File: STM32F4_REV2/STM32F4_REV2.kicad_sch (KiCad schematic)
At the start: 50 parts, among them IC1 MP2359DJ-LF-Z, J1 Screw_Terminal_01x02, J2 SWD, J3 Conn_01x04, J4 Conn_01x04, J5 USB_B_Micro, Q1 AO3401A, SW1 SW_SPDT, U1 STM32F405RGT6, U2 USBLC6-2SC6, Y1 16MHz

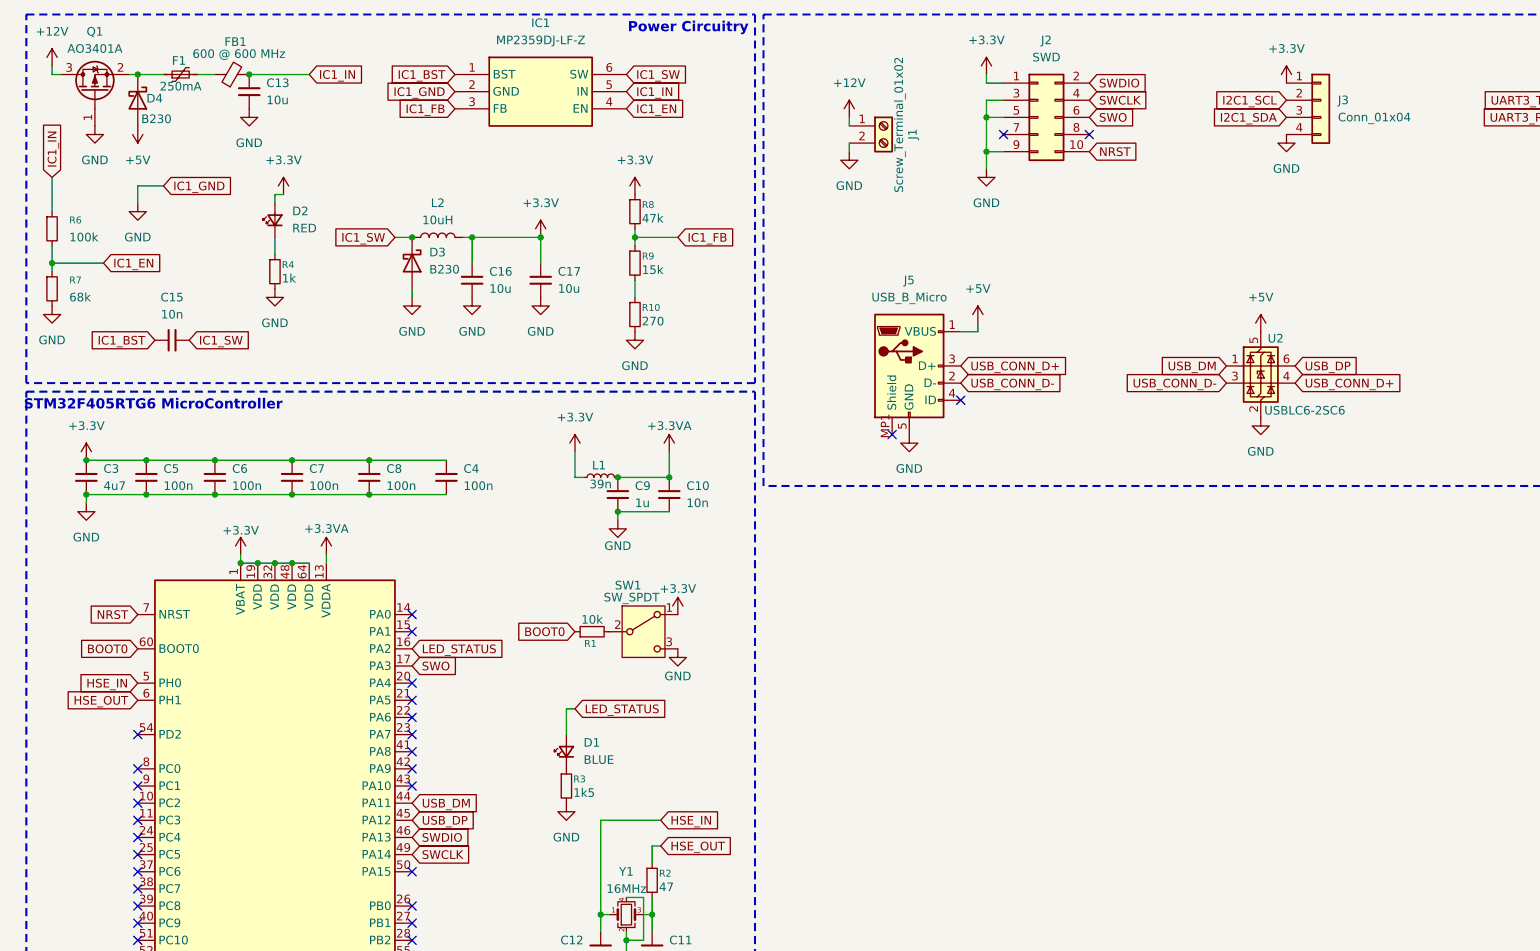
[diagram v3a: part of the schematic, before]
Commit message: Uploading the PCB files
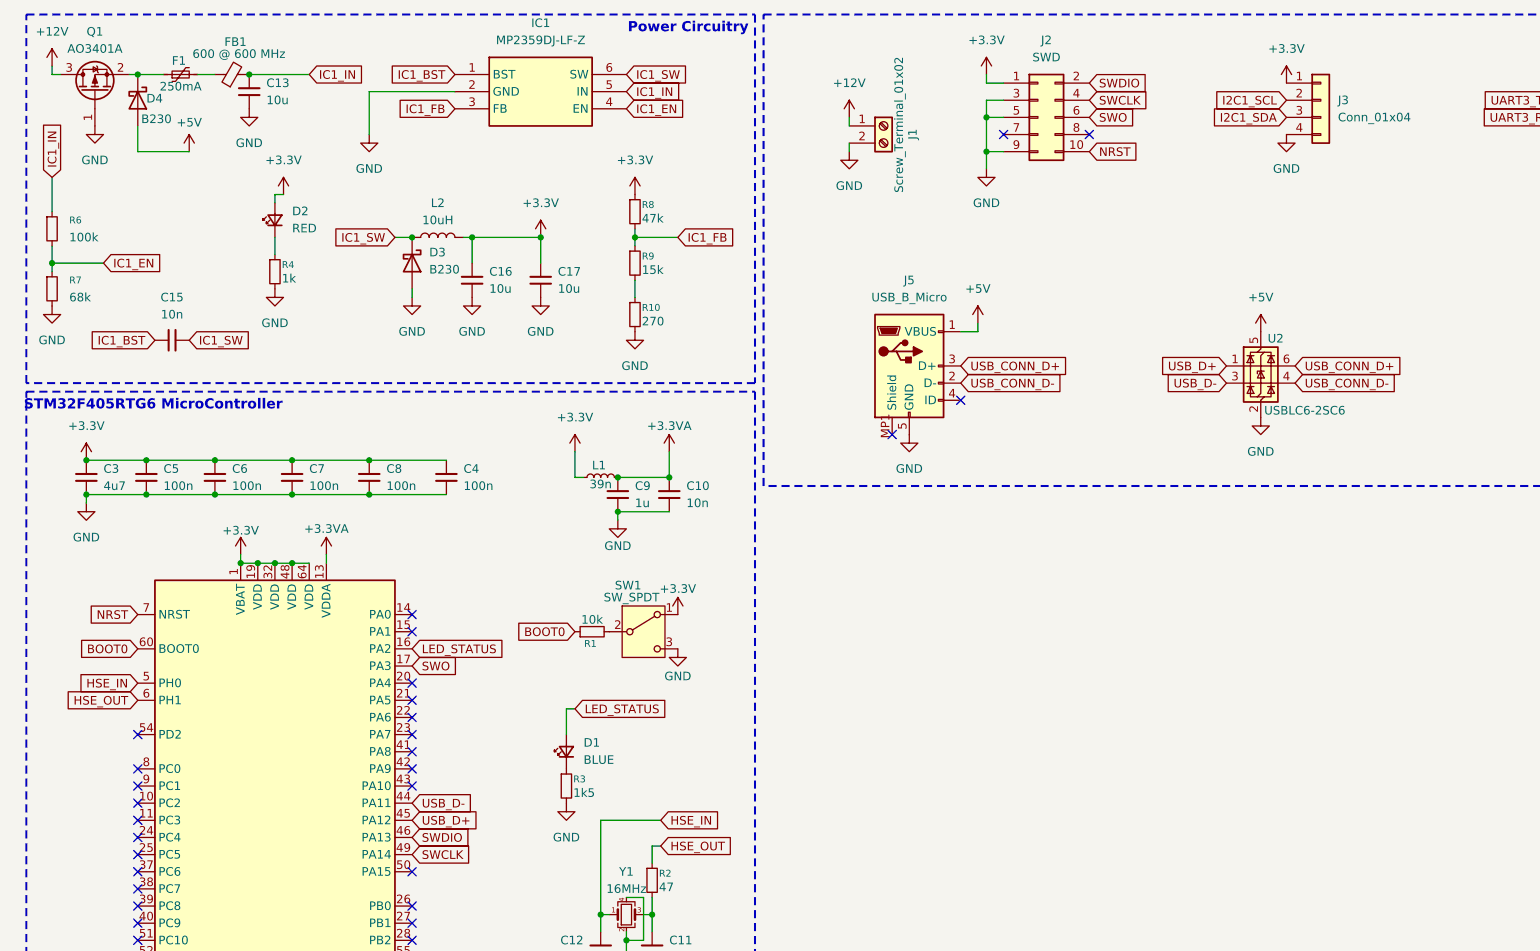
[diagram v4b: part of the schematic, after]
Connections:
- net USB_CONN_D+: now also U2.6 (I/O1); no longer U2.4 (I/O2)
- net USB_CONN_D-: now also U2.4 (I/O2); no longer U2.3 (I/O2)
- net USB_DM renamed USB_D+
- net USB_D+: now also U1.45 (PA12); no longer U1.44 (PA11)
- removed net USB_DP: U1.45 (PA12), U2.6 (I/O1)
- new net USB_D-: U1.44 (PA11), U2.3 (I/O2)
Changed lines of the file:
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@@
 	(wire
 		(pts
+			(xy 36.83 33.02) (xy 29.21 33.02)
+		)
+		(stroke
+			(width 0)
+			(type default)
+		)
+	)
+	(wire
+		(pts
 			(xy 101.6 182.88) (xy 101.6 191.77)
 		)
@@
 	(wire
 		(pts
-			(xy 29.21 38.1) (xy 29.21 40.64)
+			(xy 63.5 24.13) (xy 63.5 30.48)
 		)
 		(stroke
@@
 	(wire
 		(pts
-			(xy 33.02 38.1) (xy 29.21 38.1)
+			(xy 63.5 24.13) (xy 76.2 24.13)
 		)
 		(stroke
@@
 	(wire
 		(pts
+			(xy 29.21 33.02) (xy 29.21 29.21)
+		)
+		(stroke
+			(width 0)
+			(type default)
+		)
+	)
+	(wire
+		(pts
 			(xy 49.53 45.72) (xy 49.53 48.26)
 		)
@@
 	(global_label "USB_CONN_D-"
 		(shape input)
-		(at 190.5 67.31 180)
+		(at 200.66 67.31 0)
 		(fields_autoplaced yes)
 		(effects
@@
 				(size 1.27 1.27)
 			)
-			(justify right)
+			(justify left)
 		)
 		(property "Intersheetrefs" "${INTERSHEET_REFS}"
-			(at 173.6657 67.31 0)
+			(at 217.4943 67.31 0)
 			(hide yes)
 			(show_name no)
@@
 					(size 1.27 1.27)
 				)
-				(justify right)
+				(justify left)
 			)
 		)
@@
 		)
 	)
-	(global_label "USB_DM"
+	(global_label "USB_D-"
 		(shape input)
 		(at 69.85 129.54 0)
@@
 		)
 		(property "Intersheetrefs" "${INTERSHEET_REFS}"
-			(at 80.3342 129.54 0)
+			(at 80.4552 129.54 0)
 			(hide yes)
 			(show_name no)
@@
 		)
 	)
-	(global_label "USB_DP"
+	(global_label "USB_D+"
 		(shape input)
-		(at 200.66 64.77 0)
+		(at 190.5 64.77 180)
 		(fields_autoplaced yes)
 		(effects
@@
 				(size 1.27 1.27)
 			)
-			(justify left)
+			(justify right)
 		)
 		(property "Intersheetrefs" "${INTERSHEET_REFS}"
-			(at 210.9628 64.77 0)
+			(at 179.8948 64.77 0)
 			(hide yes)
 			(show_name no)
@@
 					(size 1.27 1.27)
 				)
-				(justify left)
+				(justify right)
 			)
 		)
@@
 		)
 	)
-	(global_label "USB_DM"
+	(global_label "USB_D-"
 		(shape input)
-		(at 190.5 64.77 180)
+		(at 190.5 67.31 180)
 		(fields_autoplaced yes)
 		(effects
@@
 		)
 		(property "Intersheetrefs" "${INTERSHEET_REFS}"
-			(at 180.0158 64.77 0)
+			(at 179.8948 67.31 0)
 			(hide yes)
 			(show_name no)
@@
 		)
 	)
-	(global_label "USB_DP"
+	(global_label "USB_D+"
 		(shape input)
 		(at 69.85 132.08 0)
@@
 		)
 		(property "Intersheetrefs" "${INTERSHEET_REFS}"
-			(at 80.1528 132.08 0)
+			(at 80.4552 132.08 0)
 			(hide yes)
 			(show_name no)
@@
 		)
 	)
-	(global_label "IC1_GND"
-		(shape input)
-		(at 76.2 24.13 180)
-		(fields_autoplaced yes)
-		(effects
-			(font
-				(size 1.27 1.27)
-			)
-			(justify right)
-		)
-		(property "Intersheetrefs" "${INTERSHEET_REFS}"
-			(at 65.2924 24.13 0)
-			(hide yes)
-			(show_name no)
-			(do_not_autoplace no)
-			(effects
-				(font
-					(size 1.27 1.27)
-				)
-				(justify right)
-			)
-		)
-	)
 	(global_label "LED_STATUS"
 		(shape input)
@@
 	(global_label "USB_CONN_D+"
 		(shape input)
-		(at 200.66 67.31 0)
+		(at 200.66 64.77 0)
 		(fields_autoplaced yes)
 		(effects
@@
 		)
 		(property "Intersheetrefs" "${INTERSHEET_REFS}"
-			(at 217.4943 67.31 0)
+			(at 217.4943 64.77 0)
 			(hide yes)
 			(show_name no)
@@
 		)
 	)
-	(global_label "IC1_GND"
-		(shape input)
-		(at 33.02 38.1 0)
-		(fields_autoplaced yes)
-		(effects
-			(font
-				(size 1.27 1.27)
-			)
-			(justify left)
-		)
-		(property "Intersheetrefs" "${INTERSHEET_REFS}"
-			(at 43.9276 38.1 0)
-			(hide yes)
-			(show_name no)
-			(do_not_autoplace no)
-			(effects
-				(font
-					(size 1.27 1.27)
-				)
-				(justify left)
-			)
-		)
-	)
 	(global_label "IC1_BST"
 		(shape input)
@@
 	(symbol
 		(lib_id "power:GND")
-		(at 29.21 40.64 0)
+		(at 63.5 30.48 0)
 		(unit 1)
 		(body_style 1)
@@
 		(fields_autoplaced yes)
 		(property "Reference" "#PWR016"
-			(at 29.21 46.99 0)
+			(at 63.5 36.83 0)
 			(hide yes)
 			(show_name no)
@@
 		)
 		(property "Value" "GND"
-			(at 29.21 45.72 0)
+			(at 63.5 35.56 0)
 			(show_name no)
 			(do_not_autoplace no)
@@
 		)
 		(property "Footprint" ""
-			(at 29.21 40.64 0)
+			(at 63.5 30.48 0)
 			(hide yes)
 			(show_name no)
@@
 		)
 		(property "Datasheet" ""
-			(at 29.21 40.64 0)
+			(at 63.5 30.48 0)
 			(hide yes)
 			(show_name no)
@@
 		)
 		(property "Description" "Power symbol creates a global label with name \"GND\" , ground"
-			(at 29.21 40.64 0)
+			(at 63.5 30.48 0)
 			(hide yes)
 			(show_name no)
@@
 	(symbol
 		(lib_id "power:+5V")
-		(at 29.21 29.21 180)
+		(at 36.83 33.02 0)
 		(unit 1)
 		(body_style 1)
@@
 		(in_pos_files yes)
 		(dnp no)
-		(fields_autoplaced yes)
 		(property "Reference" "#PWR038"
-			(at 29.21 25.4 0)
+			(at 36.83 36.83 0)
 			(hide yes)
 			(show_name no)
@@
 		)
 		(property "Value" "+5V"
-			(at 29.21 34.29 0)
+			(at 36.83 28.702 0)
 			(show_name no)
 			(do_not_autoplace no)
@@
 		)
 		(property "Footprint" ""
-			(at 29.21 29.21 0)
+			(at 36.83 33.02 0)
 			(hide yes)
 			(show_name no)
@@
 		)
 		(property "Datasheet" ""
-			(at 29.21 29.21 0)
+			(at 36.83 33.02 0)
 			(hide yes)
 			(show_name no)
@@
 		)
 		(property "Description" "Power symbol creates a global label with name \"+5V\""
-			(at 29.21 29.21 0)
+			(at 36.83 33.02 0)
 			(hide yes)
 			(show_name no)

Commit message: Uploading the PCB files kanboard #7406
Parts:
- added C17: 100n, Capacitor_SMD:C_0402_1005Metric, symbol Device:C_Small
- added J6, J7: Conn_01x04, Connector_PinHeader_2.54mm:PinHeader_1x04_P2.54mm_Vertical, symbol Connector_Generic:Conn_01x04
- added LED1: SML-LXT0805SIUGUBW, SMLLXT0805SIUGUBW, symbol DownloadedLib:SML-LXT0805SIUGUBW
- added Q2, Q3, Q4: 2N7002K, Package_TO_SOT_SMD:SOT-23, symbol Transistor_FET:2N7002K
- added R5: 10k, Resistor_SMD:R_0603_1608Metric, symbol Device:R_Small
- added SW2: SW_Push, Button_Switch_THT:SW_PUSH_6mm_H5mm, symbol Switch:SW_Push
- added TP1, TP2, TP3, TP4: TestPoint, TestPoint:TestPoint_Pad_D1.5mm, symbol Connector:TestPoint
- R11: value 2k2 -> 4k7; Field5 (none) -> 4.7 kΩ, ±5%, 0.125 W
- R12: value 2k2 -> 4k7
- renumbered C15 to C14, C16 to C15, C17 to C16, D1 to STATUS1
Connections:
- net +3.3V: now also R5.1, TP2.1
- net +3.3VA: now also TP1.1
- net GND: now also C17.2, J6.3 (Pin_3), J7.3 (Pin_3), SW2.1, TP3.1
- net I2C1_SCL: now also J7.1 (Pin_1)
- net I2C1_SDA: now also J7.2 (Pin_2)
- net NRST: now also C17.1, R5.2, SW2.2, TP4.1; no longer J2.10 (Pin_10)
- net SWO: now also U1.55 (PB3); no longer U1.17 (PA3)
- net UART3_RX: now also J6.2 (Pin_2)
- net UART3_TX: now also J6.1 (Pin_1)
- no-connect marks 43 -> 44
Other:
- note added: "Test Points"
- note removed: "Cload = 2 * (CL - Cstray)"
- moved on the sheet: C13, C14, C15, C16, D2, D3, D4, F1, FB1, H1, H2, H3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
